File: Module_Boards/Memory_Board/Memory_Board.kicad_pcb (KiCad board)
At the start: 6 copper layers, 10.8 x 15.2 mm, 17 parts, among them U1 MX25U12832FZNI02-TR, U2 MX25U25643GZ4I00-T

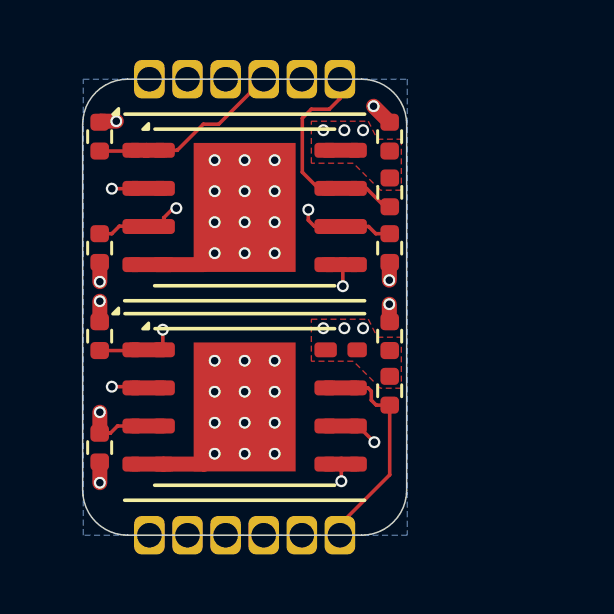
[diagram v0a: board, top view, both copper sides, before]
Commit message: Big push. Fixed the issues that were pending. See github
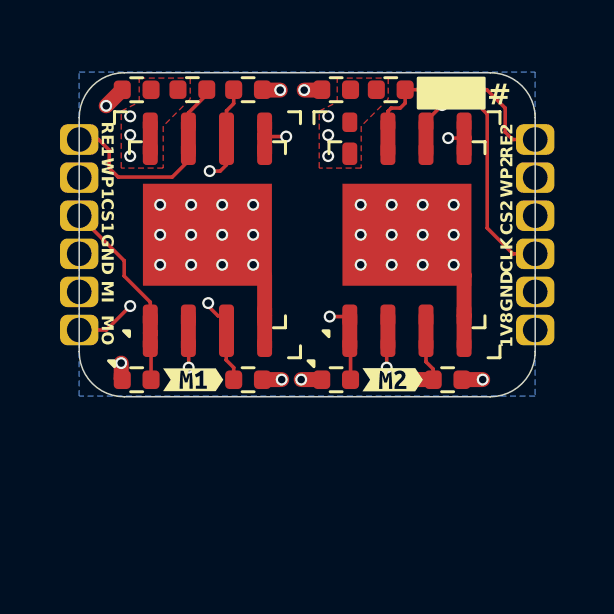
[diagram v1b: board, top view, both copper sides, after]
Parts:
- added kibuzzard-6743EB85: G***, kibuzzard-6743EB85, F.Cu at (148.1, 100.2)
- added kibuzzard-6743EB8D: G***, kibuzzard-6743EB8D, F.Cu at (154.7, 100.2)
- moved R7 11.8 mm to (156.5, 100.2), turned to 180 degrees
- moved kibuzzard-672506D5 11.7 mm to (157.9, 95.4), turned to -90 degrees
- moved R8 10.0 mm to (154.6, 90.5), turned to 0 degrees
- moved C1 8.58 mm to (146.2, 90.6), turned to 180 degrees
- moved C2 8.41 mm to (152.8, 90.5), turned to 180 degrees
- moved R1 8.20 mm to (146.2, 100.2), turned to 0 degrees
- moved R5 8.02 mm to (152.8, 100.2), turned to 0 degrees
- moved U2 7.89 mm to (155.2, 95.4), turned to 90 degrees
- moved G*** 7.71 mm to (155.1, 95.4), turned to -90 degrees
- moved R4 7.42 mm to (148.0, 90.5), turned to 0 degrees
- moved R2 7.08 mm to (149.9, 90.5), turned to 180 degrees
- moved R3 6.61 mm to (149.9, 100.2), turned to 180 degrees
- moved G*** 4.18 mm to (146.7, 95.7), turned to -90 degrees
- moved J1 3.19 mm to (151.9, 95.4), turned to 180 degrees
- moved kibuzzard-672506E3 2.37 mm to (151.3, 95.7), turned to -90 degrees
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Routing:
- net FLASH_CLK: track 24.1 -> 21.9 mm
- net FLASH_MOSI_(IO0): track 22.9 -> 23.6 mm, vias 2 -> 3
- added copper zone on In4.Cu, net GND
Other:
- board size 10.8 x 15.2 mm -> 15.2 x 10.8 mm
- board text added: "#"
- board text added: "1V8"
- board text added: "CLK"
- board text added: "CS1"
- board text added: "CS2"
- board text added: "GND"
- board text added: "MI"
- board text added: "MO"
- board text added: "RE1"
- board text added: "RE2"
- board text added: "WP1"
- board text added: "WP2"
